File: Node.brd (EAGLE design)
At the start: 27.9 x 27.9 mm, 60 parts, among them J1 DF12A3.0-14DS, Q1 16MHz, U1 ATMEGA32U4QFN, U2 NRF24L01NOPAD, U3 LTC3553, U4 L3GD20, U6 LSM303DLHC, U7 BD2425NNRF0404, U9 RCLAMP0502A, X1 USB-FCI

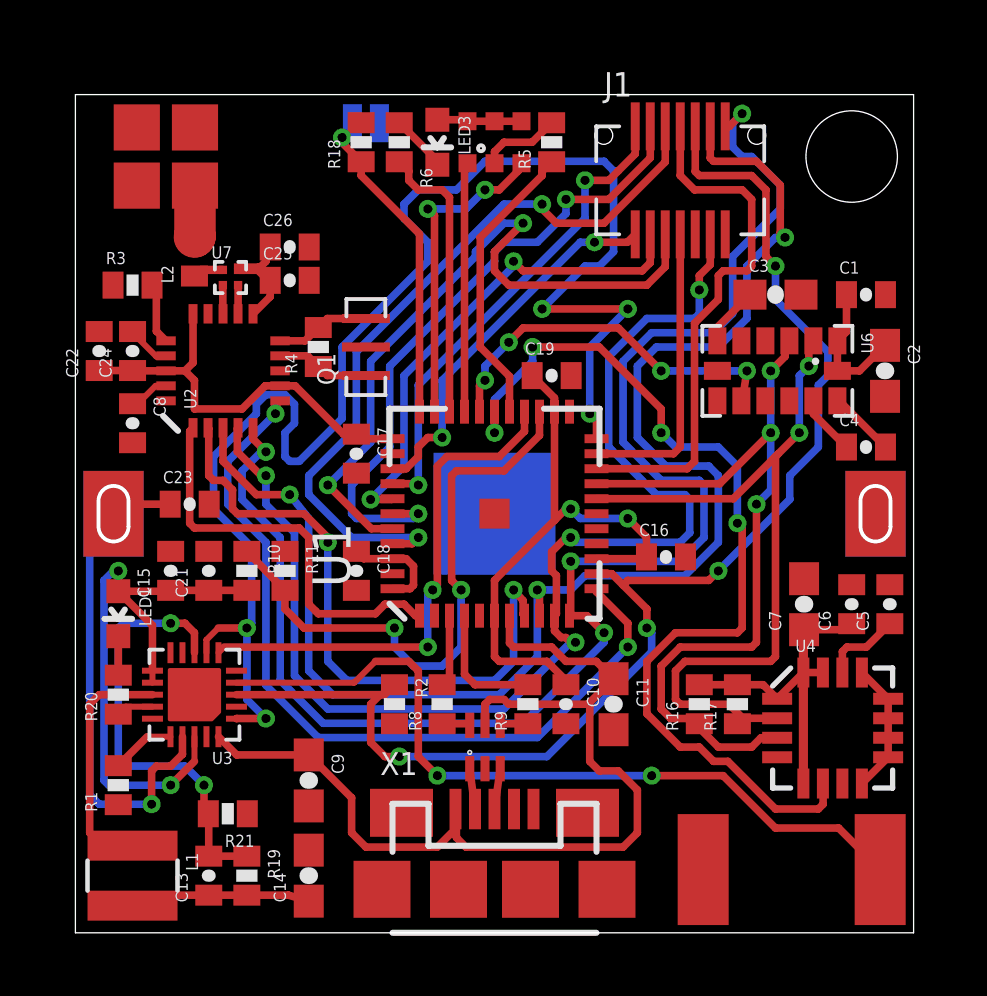
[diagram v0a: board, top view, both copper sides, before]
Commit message: so close
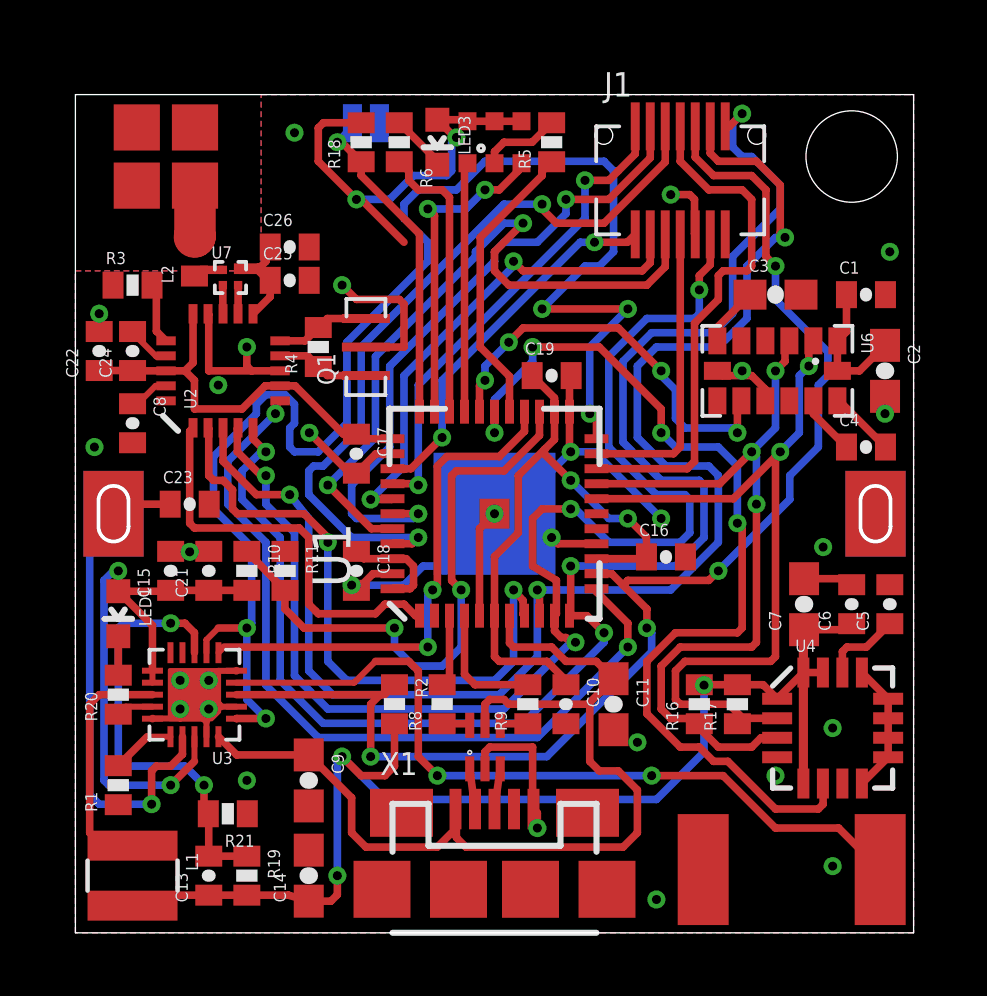
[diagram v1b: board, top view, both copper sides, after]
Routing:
- net GND: track 5.92 -> 61.8 mm, vias 0 -> 29
- net +3V3: track 61.7 -> 100.0 mm, vias 2 -> 7
- net MOSI: track 42.4 -> 44.9 mm
- net PCINT5: track 12.5 -> 13.8 mm
- net SDA: track 26.6 -> 25.8 mm
- added copper zone on layer 1, net GND
- added copper zone on layer 16, net GND
